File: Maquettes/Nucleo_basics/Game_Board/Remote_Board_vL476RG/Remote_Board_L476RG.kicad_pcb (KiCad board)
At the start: 2 copper layers, 199 x 123 mm, 47 parts, among them CON1 MikroE-nRF-S-module, J1 LCD_SD, J10 3.3V_reg, J2 JoyStick, J3 AnalogIn, J4 BAT_IN, J5 Morpho_Gauche, J6 Morpho_Droite, J7 I2C_Visu, J8 I2C_EXT, J9 GND_reg, SW1 SW_1, SW2 SW_2, SW3 SW_3, SW4 SW_4, SW5 SW_5, U1 MCP23008-xP

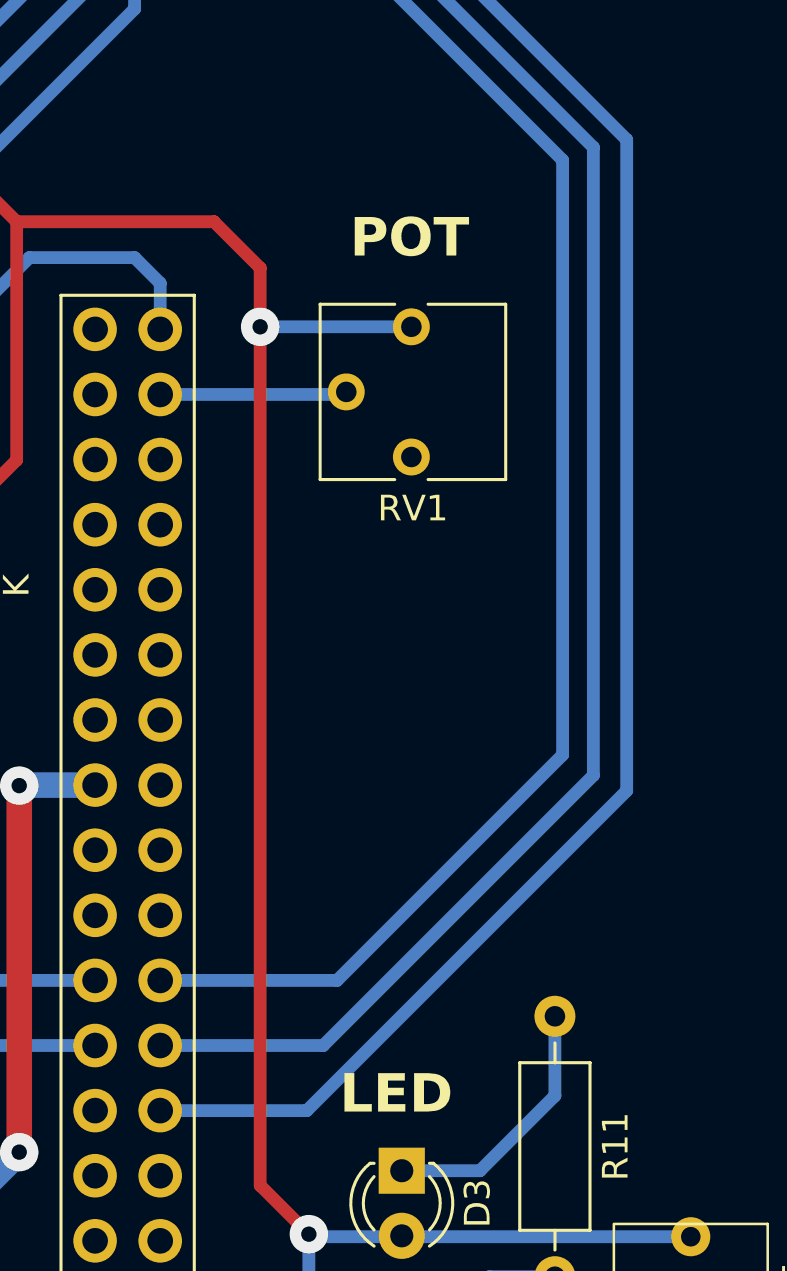
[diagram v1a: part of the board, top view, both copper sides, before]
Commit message: Update Remote and Robot Boards
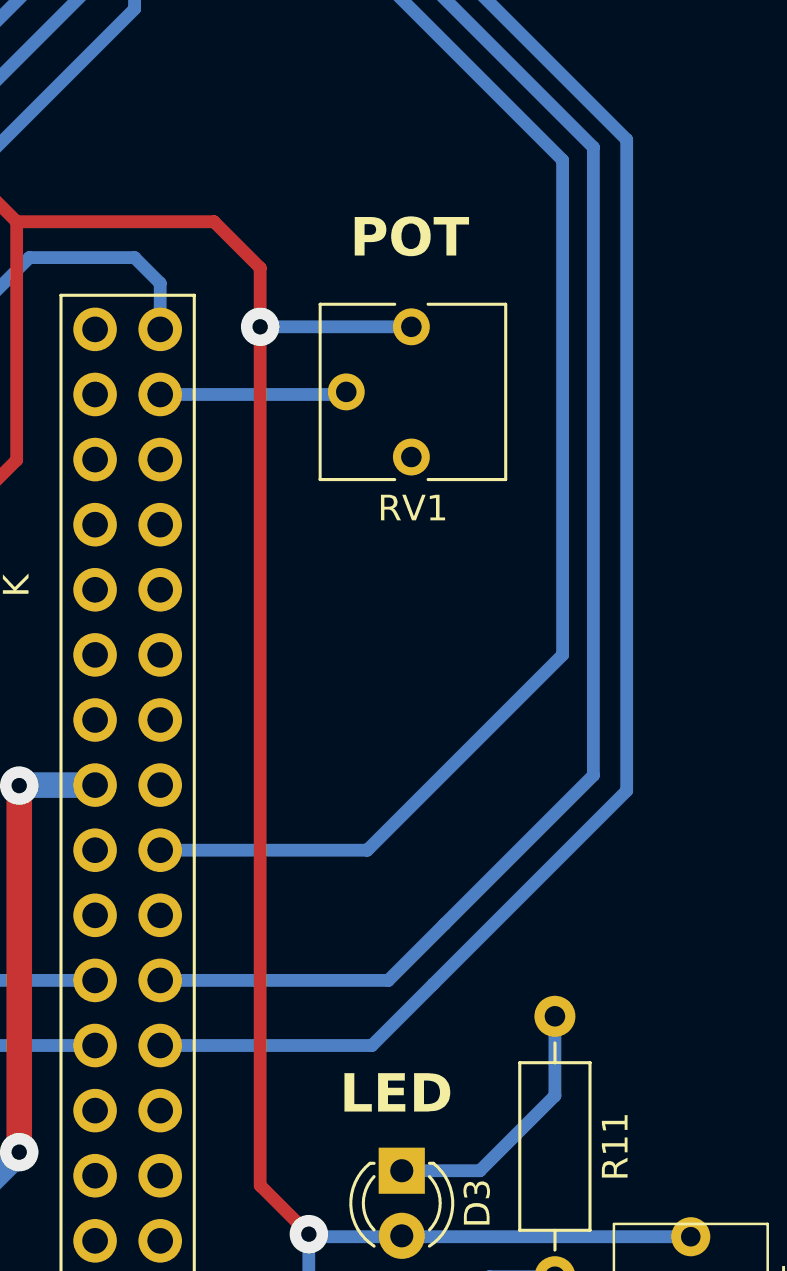
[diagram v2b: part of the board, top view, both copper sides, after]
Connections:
- J5 pad 15: nRF_INT -> unconnected-(J5-Pin_15-Pad15)
- J5 pad 17: nRF_CE -> nRF_INT
- J5 pad 19: nRF_CS -> nRF_CE
- J5 pad 23: unconnected-(J5-Pin_23-Pad23) -> nRF_CS
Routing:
- net nRF_CS: track 89.4 -> 85.0 mm
- net nRF_INT: track 91.0 -> 89.9 mm
- net nRF_CE: track 95.6 -> 94.5 mm
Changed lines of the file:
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@@
 	(net 56 "unconnected-(J5-Pin_4-Pad4)")
 	(net 57 "unconnected-(J5-Pin_29-Pad29)")
-	(net 58 "unconnected-(J5-Pin_23-Pad23)")
+	(net 58 "unconnected-(J5-Pin_15-Pad15)")
 	(net 59 "POT_OUT")
 	(net 60 "unconnected-(J6-Pin_19-Pad19)")
@@
 			(layers "*.Cu" "*.Mask")
 			(remove_unused_layers no)
-			(net 14 "nRF_INT")
+			(net 58 "unconnected-(J5-Pin_15-Pad15)")
 			(pinfunction "Pin_15")
 			(pintype "passive")
@@
 			(layers "*.Cu" "*.Mask")
 			(remove_unused_layers no)
-			(net 13 "nRF_CE")
+			(net 14 "nRF_INT")
 			(pinfunction "Pin_17")
 			(pintype "passive")
@@
 			(layers "*.Cu" "*.Mask")
 			(remove_unused_layers no)
-			(net 9 "nRF_CS")
+			(net 13 "nRF_CE")
 			(pinfunction "Pin_19")
 			(pintype "passive")
@@
 			(layers "*.Cu" "*.Mask")
 			(remove_unused_layers no)
-			(net 58 "unconnected-(J5-Pin_23-Pad23)")
+			(net 9 "nRF_CS")
 			(pinfunction "Pin_23")
 			(pintype "passive")
@@
 	)
 	(segment
-		(start 220.6 74.6)
-		(end 232.9 86.9)
+		(start 217.2 113.82)
+		(end 225.28 113.82)
 		(width 0.5)
 		(layer "B.Cu")
@@
 	)
 	(segment
-		(start 219.11 57.21)
-		(end 220.6 58.7)
+		(start 232.9 86.9)
+		(end 232.9 106.2)
 		(width 0.5)
 		(layer "B.Cu")
@@
 	)
 	(segment
-		(start 207.67 57.21)
-		(end 219.11 57.21)
+		(start 220.6 74.6)
+		(end 232.9 86.9)
 		(width 0.5)
 		(layer "B.Cu")
@@
 	)
 	(segment
-		(start 224.1 118.9)
-		(end 217.2 118.9)
+		(start 225.28 113.82)
+		(end 232.9 106.2)
 		(width 0.5)
 		(layer "B.Cu")
@@
 	)
 	(segment
-		(start 232.9 110.1)
-		(end 224.1 118.9)
+		(start 219.11 57.21)
+		(end 220.6 58.7)
 		(width 0.5)
 		(layer "B.Cu")
@@
 	)
 	(segment
-		(start 232.9 86.9)
-		(end 232.9 110.1)
+		(start 207.67 57.21)
+		(end 219.11 57.21)
 		(width 0.5)
 		(layer "B.Cu")
@@
 	)
 	(segment
+		(start 226.1 118.9)
+		(end 228.3 116.7)
+		(width 0.5)
+		(layer "B.Cu")
+		(net 13)
+	)
+	(segment
 		(start 221.8 74.1)
 		(end 221.8 56.6)
@@
 	)
 	(segment
+		(start 228.3 116.7)
+		(end 234.1 110.9)
+		(width 0.5)
+		(layer "B.Cu")
+		(net 13)
+	)
+	(segment
 		(start 219.87 54.67)
 		(end 207.67 54.67)
@@
 	)
 	(segment
-		(start 223.56 121.44)
-		(end 234.1 110.9)
-		(width 0.5)
-		(layer "B.Cu")
-		(net 13)
-	)
-	(segment
-		(start 217.2 121.44)
-		(end 223.56 121.44)
+		(start 217.2 118.9)
+		(end 226.1 118.9)
 		(width 0.5)
 		(layer "B.Cu")
@@
 	)
 	(segment
-		(start 222.92 123.98)
+		(start 227.85 119.05)
 		(end 235.4 111.5)
 		(width 0.5)
@@
 	)
 	(segment
-		(start 217.2 123.98)
-		(end 222.92 123.98)
+		(start 217.2 121.44)
+		(end 225.46 121.44)
 		(width 0.5)
 		(layer "B.Cu")
@@
 		(width 0.5)
 		(layer "B.Cu")
+		(net 14)
+	)
+	(segment
+		(start 225.46 121.44)
+		(end 227.85 119.05)
+		(width 0.5)
+		(layer "B.Cu")
